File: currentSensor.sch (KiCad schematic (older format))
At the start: 0 parts

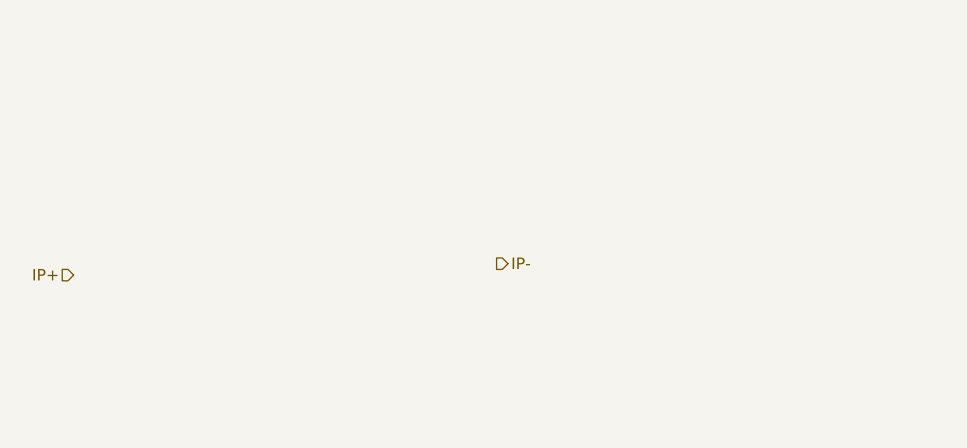
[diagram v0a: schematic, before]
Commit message: Esquemático acabado y asignación de huellas
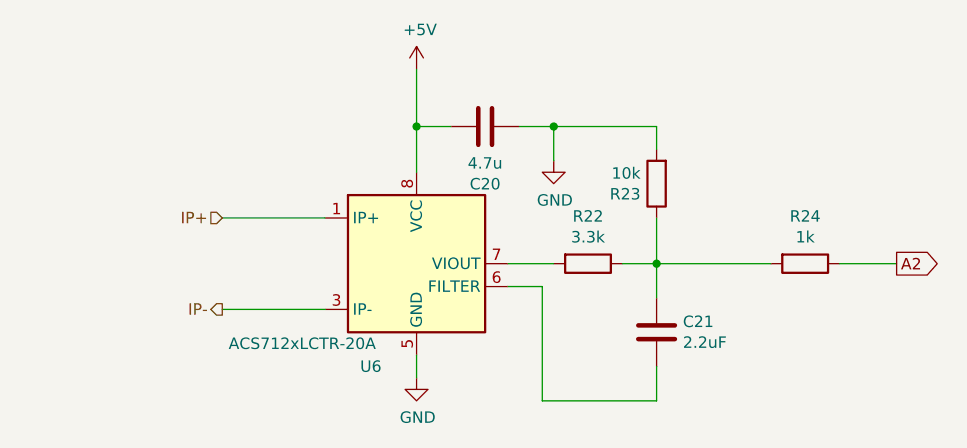
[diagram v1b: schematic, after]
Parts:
- added C20: 4.7u, Capacitors_SMD:CP_Elec_3x5.3, symbol Device:C
- added C21: 2.2uF, Capacitors_SMD:C_0603, symbol Device:C
- added R22: 3.3k, Resistors_SMD:R_0603, symbol Device:R
- added R23: 10k, Resistors_SMD:R_0603, symbol Device:R
- added R24: 1k, Resistors_SMD:R_0603, symbol Device:R
- added U6: ACS712xLCTR-20A, Housings_SOIC:SOIC-8_3.9x4.9mm_Pitch1.27mm, symbol Sensor_Current:ACS712xLCTR-20A
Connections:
- net IP+: now also U6.1 (IP+), U6.2 (IP+)
- net IP-: now also U6.3 (IP-), U6.4 (IP-)
- new net: C21.1, U6.6 (FILTER)
- new net: R22.2, U6.7 (VIOUT)
- new net: C21.2, R22.1, R23.1, R24.2
- new net +5V: C20.1, U6.8 (VCC)
- new net A2: R24.1
- new net GND: C20.2, R23.2, U6.5 (GND)
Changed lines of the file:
@@
 Comment4 ""
 $EndDescr
-Text HLabel 5900 3500 2    50   Output ~ 0
+Text HLabel 4700 3700 0    50   Output ~ 0
 IP-
-Text HLabel 4050 3550 0    50   Input ~ 0
+Text HLabel 4700 3300 0    50   Input ~ 0
 IP+
+$Comp
+L Sensor_Current:ACS712xLCTR-20A U6
+U 1 1 61C260B3
+P 5550 3500
+F 0 "U6" H 5350 3050 50  0000 C CNN
+F 1 "ACS712xLCTR-20A" H 5050 3150 50  0000 C CNN
+F 2 "Housings_SOIC:SOIC-8_3.9x4.9mm_Pitch1.27mm" H 5650 3150 50  0001 L CIN
+F 3 "http://www.allegromicro.com/~/media/Files/Datasheets/ACS712-Datasheet.ashx?la=en" H 5550 3500 50  0001 C CNN
+	1    5550 3500
+	1    0    0    -1
+$EndComp
+Wire Wire Line
+	4700 3300 5150 3300
+Wire Wire Line
+	4700 3700 5150 3700
+Wire Wire Line
+	5550 3100 5550 2900
+Wire Wire Line
+	5550 2900 5700 2900
+$Comp
+L Device:C C20
+U 1 1 61C26F1D
+P 5850 2900
+F 0 "C20" V 5598 2900 50  0000 C CNN
+F 1 "4.7u" V 5689 2900 50  0000 C CNN
+F 2 "Capacitors_SMD:CP_Elec_3x5.3" H 5888 2750 50  0001 C CNN
+F 3 "~" H 5850 2900 50  0001 C CNN
+	1    5850 2900
+	0    -1   -1   0
+$EndComp
+$Comp
+L power:GND #PWR022
+U 1 1 61C27599
+P 6150 3050
+F 0 "#PWR022" H 6150 2800 50  0001 C CNN
+F 1 "GND" H 6155 2877 50  0000 C CNN
+F 2 "" H 6150 3050 50  0001 C CNN
+F 3 "" H 6150 3050 50  0001 C CNN
+	1    6150 3050
+	1    0    0    -1
+$EndComp
+$Comp
+L power:GND #PWR021
+U 1 1 61C29222
+P 5550 4000
+F 0 "#PWR021" H 5550 3750 50  0001 C CNN
+F 1 "GND" H 5555 3827 50  0000 C CNN
+F 2 "" H 5550 4000 50  0001 C CNN
+F 3 "" H 5550 4000 50  0001 C CNN
+	1    5550 4000
+	1    0    0    -1
+$EndComp
+Wire Wire Line
+	5550 4000 5550 3900
+Wire Wire Line
+	6000 2900 6150 2900
+Wire Wire Line
+	6150 2900 6150 3050
+Wire Wire Line
+	5550 2900 5550 2650
+Connection ~ 5550 2900
+$Comp
+L power:+5V #PWR020
+U 1 1 61C2A74C
+P 5550 2650
+F 0 "#PWR020" H 5550 2500 50  0001 C CNN
+F 1 "+5V" H 5565 2823 50  0000 C CNN
+F 2 "" H 5550 2650 50  0001 C CNN
+F 3 "" H 5550 2650 50  0001 C CNN
+	1    5550 2650
+	1    0    0    -1
+$EndComp
+$Comp
+L Device:R R23
+U 1 1 61C2AB8D
+P 6600 3150
+F 0 "R23" H 6670 3196 50  0000 L CNN
+F 1 "10k" H 6670 3105 50  0000 L CNN
+F 2 "Resistors_SMD:R_0603" V 6530 3150 50  0001 C CNN
+F 3 "~" H 6600 3150 50  0001 C CNN
+	1    6600 3150
+	-1   0    0    1
+$EndComp
+$Comp
+L Device:R R22
+U 1 1 61C2ACF9
+P 6300 3500
+F 0 "R22" V 6093 3500 50  0000 C CNN
+F 1 "3.3k" V 6184 3500 50  0000 C CNN
+F 2 "Resistors_SMD:R_0603" V 6230 3500 50  0001 C CNN
+F 3 "~" H 6300 3500 50  0001 C CNN
+	1    6300 3500
+	0    1    1    0
+$EndComp
+Wire Wire Line
+	5950 3500 6150 3500
+Wire Wire Line
+	6450 3500 6600 3500
+Wire Wire Line
+	6600 3300 6600 3500
+Wire Wire Line
+	6600 3000 6600 2900
+Wire Wire Line
+	6600 2900 6150 2900
+Connection ~ 6150 2900
+Connection ~ 6600 3500
+Wire Wire Line
+	6600 4100 6600 3950
+$Comp
+L Device:C C21
+U 1 1 61C2CBB3
+P 6600 3800
+F 0 "C21" H 6485 3754 50  0000 R CNN
+F 1 "2.2uF" H 6485 3845 50  0000 R CNN
+F 2 "Capacitors_SMD:C_0603" H 6638 3650 50  0001 C CNN
+F 3 "~" H 6600 3800 50  0001 C CNN
+	1    6600 3800
+	-1   0    0    1
+$EndComp
+Wire Wire Line
+	6600 3650 6600 3500
+$Comp
+L Device:R R24
+U 1 1 61C2D83A
+P 7250 3500
+F 0 "R24" V 7043 3500 50  0000 C CNN
+F 1 "1k" V 7134 3500 50  0000 C CNN
+F 2 "Resistors_SMD:R_0603" V 7180 3500 50  0001 C CNN
+F 3 "~" H 7250 3500 50  0001 C CNN
+	1    7250 3500
+	0    1    1    0
+$EndComp
+Wire Wire Line
+	7400 3500 7650 3500
+Text GLabel 7650 3500 2    50   Output ~ 0
+A2
+Wire Wire Line
+	6600 3500 7100 3500
+Wire Wire Line
+	6600 4100 6100 4100
+Wire Wire Line
+	6100 4100 6100 3600
+Wire Wire Line
+	6100 3600 5950 3600
 $EndSCHEMATC
